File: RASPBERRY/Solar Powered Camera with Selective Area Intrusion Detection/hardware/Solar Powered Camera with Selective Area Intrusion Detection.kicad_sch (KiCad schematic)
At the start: 0 parts

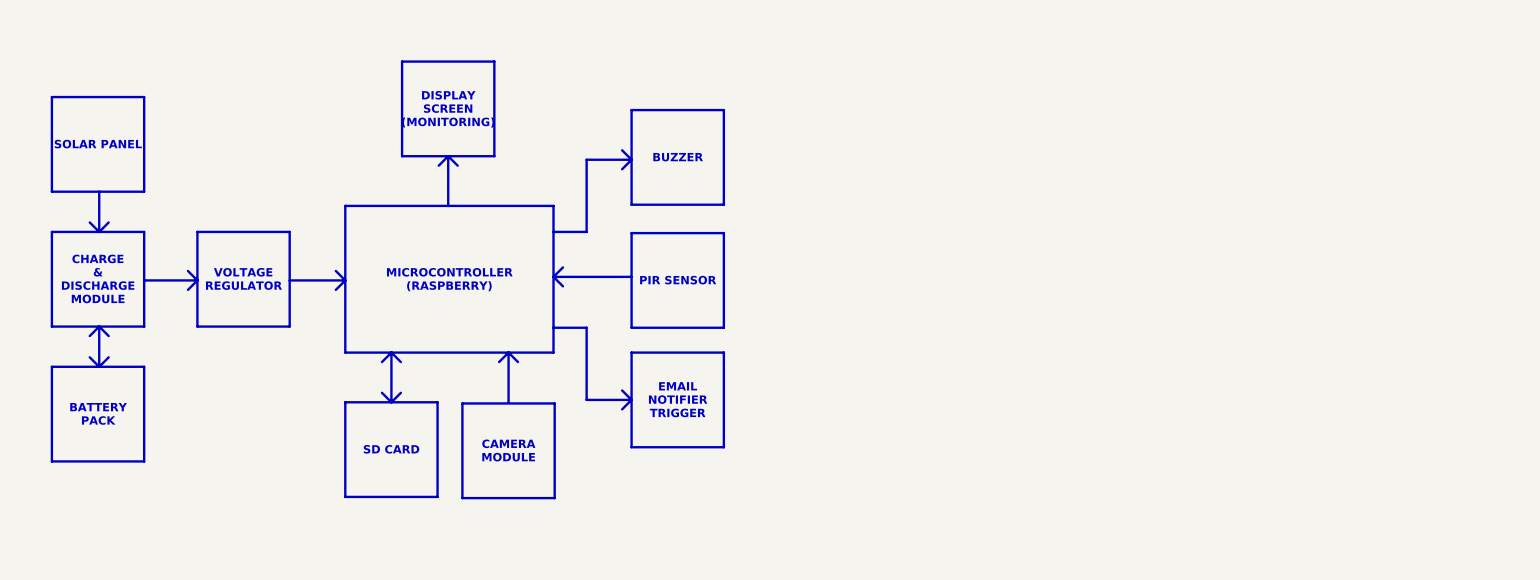
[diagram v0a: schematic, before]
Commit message: update from home
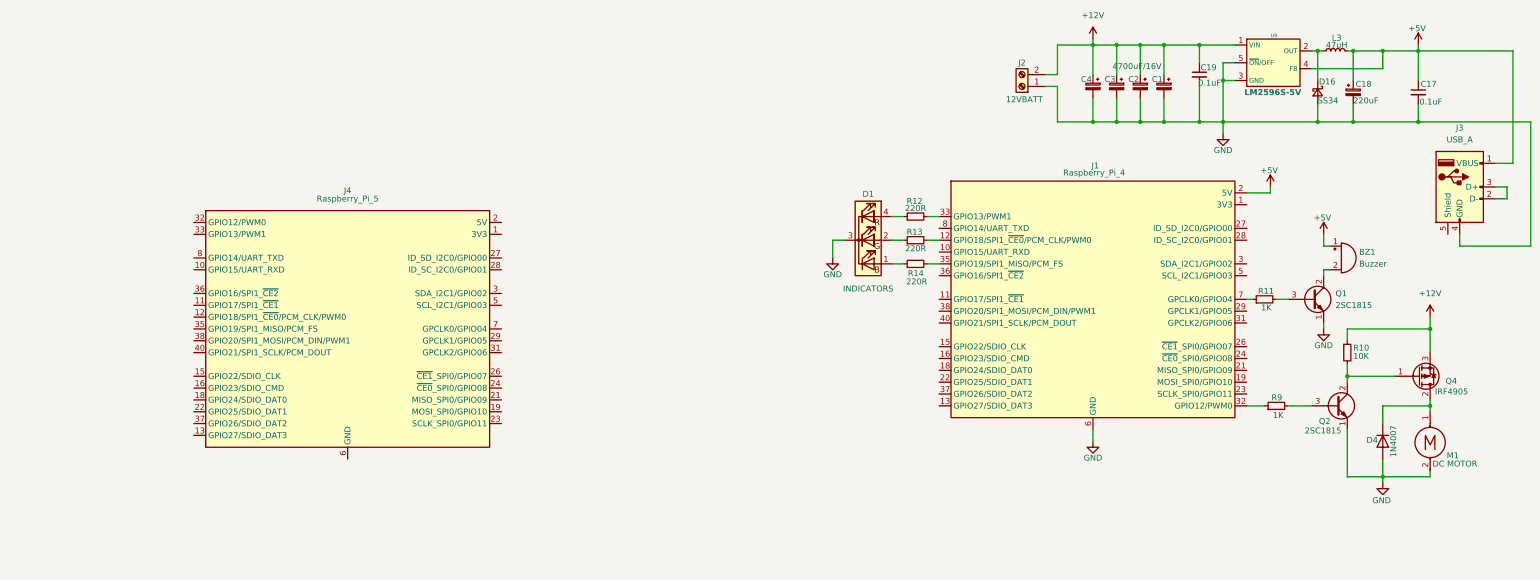
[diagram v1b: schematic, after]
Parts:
- added BZ1: Buzzer, Buzzer_Beeper:Buzzer_12x9.5RM7.6, symbol Device:Buzzer
- added C1: 4700uF/16V, Capacitor_THT:CP_Radial_D13.0mm_P5.00mm, symbol Device:C_Polarized_Small
- added C17, C19: 0.1uF, Capacitor_THT:C_Disc_D7.5mm_W5.0mm_P7.50mm, symbol Device:C_Small
- added C18: 220uF, Capacitor_THT:CP_Radial_D8.0mm_P3.50mm, symbol Device:C_Polarized_Small
- added C2, C3, C4: ~, Capacitor_THT:CP_Radial_D13.0mm_P5.00mm, symbol Device:C_Polarized_Small
- added D1: INDICATORS, LED_THT:LED_D5.0mm-4_RGB, symbol Device:LED_BGKR
- added D16: SS34, Diode_SMD:D_3220_8050Metric, symbol Device:D_Schottky_Small
- added D4: 1N4007, Diode_THT:D_DO-41_SOD81_P10.16mm_Horizontal, symbol Diode:1N4007
- added J1: Raspberry_Pi_4, Connector_PinHeader_2.54mm:PinHeader_2x20_P2.54mm_Vertical, symbol Connector:Raspberry_Pi_4
- added J2: 12VBATT, TerminalBlock_4Ucon:TerminalBlock_4Ucon_1x02_P3.50mm_Vertical, symbol Connector:Screw_Terminal_01x02
- added J3: USB_A, Connector_USB:USB_A_Molex_67643_Horizontal, symbol Connector:USB_A
- added J4: Raspberry_Pi_5, symbol Connector:Raspberry_Pi_4
- added L3: 47uH, Inductor_THT:L_Axial_L14.0mm_D4.5mm_P15.24mm_Horizontal_Fastron_LACC, symbol Device:L_Small
- added M1: DC MOTOR, TerminalBlock_4Ucon:TerminalBlock_4Ucon_1x02_P3.50mm_Vertical, symbol Motor:Motor_AC
- added Q1, Q2: 2SC1815, Package_TO_SOT_THT:TO-92S_Wide, symbol Transistor_BJT:2SC1815
- added Q4: IRF4905, Package_TO_SOT_THT:TO-220-3_Horizontal_TabDown, symbol Transistor_FET:IRF4905
- added R10: 10K, Resistor_THT:R_Axial_DIN0207_L6.3mm_D2.5mm_P10.16mm_Horizontal, symbol Device:R_Small
- added R11, R9: 1K, Resistor_THT:R_Axial_DIN0207_L6.3mm_D2.5mm_P10.16mm_Horizontal, symbol Device:R_Small
- added R12, R13, R14: 220R, Resistor_THT:R_Axial_DIN0207_L6.3mm_D2.5mm_P10.16mm_Horizontal, symbol Device:R_Small
- added U9: LM2596S-5V, Package_TO_SOT_SMD:TO-263-5_TabPin3, symbol Regulator_Switching:LM2596S-ADJ
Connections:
- new net: D16.1 (K), L3.1, U9.2 (OUT)
- new net: Q2.2 (C), Q4.1 (G), R10.2
- new net: J1.7 (GPCLK0/GPIO04), R11.1
- new net: Q1.3 (B), R11.2
- new net: D1.2 (GA), R13.1
- new net: J1.12 (GPIO18/SPI1_~{CE0}/PCM_CLK/PWM0), R13.2
- new net: J1.32 (GPIO12/PWM0), R9.1
- new net: Q2.3 (B), R9.2
- new net: D4.1 (K), M1.1, Q4.2 (D)
- new net: J3.2 (D-), J3.3 (D+)
- new net: BZ1.2 (-), Q1.2 (C)
- new net: D1.4 (RA), R12.1
- new net: J1.33 (GPIO13/PWM1), R12.2
- new net: J1.1 (3V3), J1.17 (3V3)
- new net: J1.35 (GPIO19/SPI1_MISO/PCM_FS), R14.2
- new net: J4.1 (3V3), J4.17 (3V3)
- new net: J4.14 (GND), J4.20 (GND), J4.25 (GND), J4.30 (GND), J4.34 (GND), J4.39 (GND), J4.6 (GND), J4.9 (GND)
- new net: J4.2 (5V), J4.4 (5V)
- new net: D1.1 (BA), R14.1
- new net +12V: C1.1, C19.1, C2.1, C3.1, C4.1, J2.2 (Pin_2), Q4.3 (S), R10.1, U9.1 (VIN)
- new net +5V: BZ1.1 (+), C17.1, C18.1, J1.2 (5V), J1.4 (5V), J3.1 (VBUS), L3.2, U9.4 (FB)
- new net GND: C1.2, C17.2, C18.2, C19.2, C2.2, C3.2, C4.2, D1.3 (K), D16.2 (A), D4.2 (A), J1.14 (GND), J1.20 (GND), J1.25 (GND), J1.30 (GND), J1.34 (GND), J1.39 (GND), J1.6 (GND), J1.9 (GND), J2.1 (Pin_1), J3.4 (GND), M1.2, Q1.1 (E), Q2.1 (E), U9.3 (GND), U9.5 (~{ON}/OFF)

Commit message: UPDATED
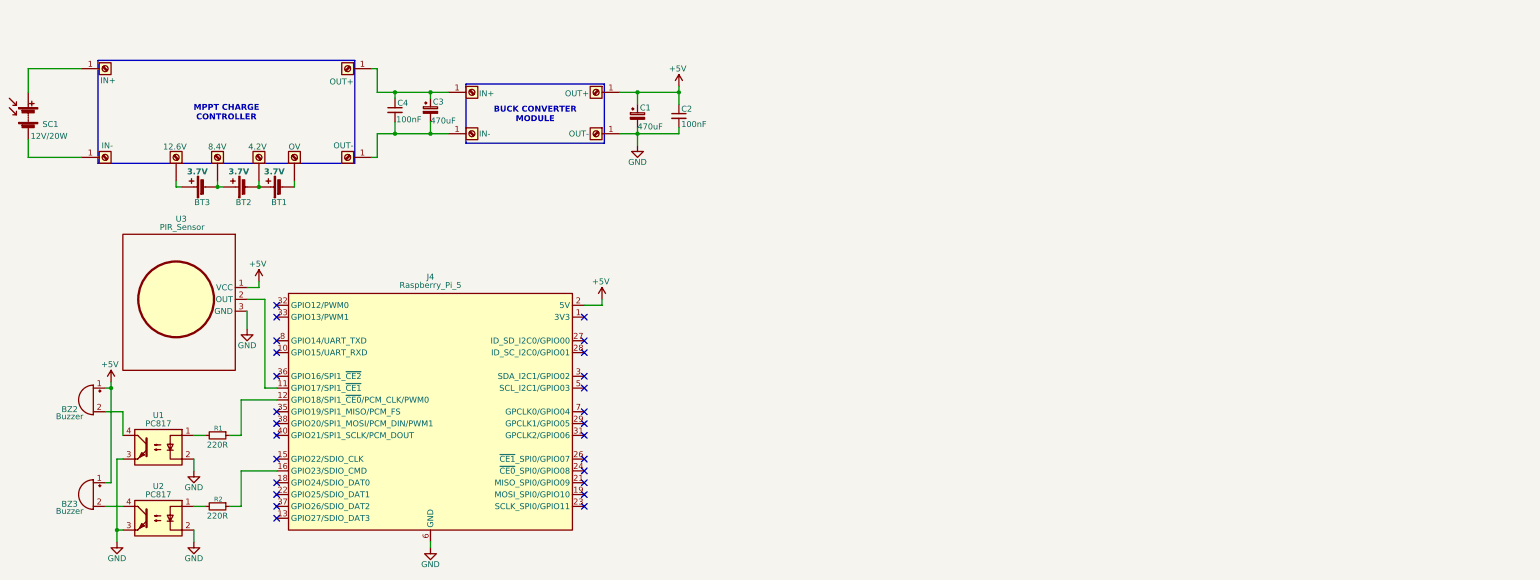
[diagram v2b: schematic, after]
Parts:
- removed BZ1: Buzzer, Buzzer_Beeper:Buzzer_12x9.5RM7.6, symbol Device:Buzzer
- removed C17, C19: 0.1uF, Capacitor_THT:C_Disc_D7.5mm_W5.0mm_P7.50mm, symbol Device:C_Small
- removed C18: 220uF, Capacitor_THT:CP_Radial_D8.0mm_P3.50mm, symbol Device:C_Polarized_Small
- removed C2, C4: ~, Capacitor_THT:CP_Radial_D13.0mm_P5.00mm, symbol Device:C_Polarized_Small
- removed D1: INDICATORS, LED_THT:LED_D5.0mm-4_RGB, symbol Device:LED_BGKR
- removed D16: SS34, Diode_SMD:D_3220_8050Metric, symbol Device:D_Schottky_Small
- removed D4: 1N4007, Diode_THT:D_DO-41_SOD81_P10.16mm_Horizontal, symbol Diode:1N4007
- removed J1: Raspberry_Pi_4, Connector_PinHeader_2.54mm:PinHeader_2x20_P2.54mm_Vertical, symbol Connector:Raspberry_Pi_4
- removed J2: 12VBATT, TerminalBlock_4Ucon:TerminalBlock_4Ucon_1x02_P3.50mm_Vertical, symbol Connector:Screw_Terminal_01x02
- removed J3: USB_A, Connector_USB:USB_A_Molex_67643_Horizontal, symbol Connector:USB_A
- removed L3: 47uH, Inductor_THT:L_Axial_L14.0mm_D4.5mm_P15.24mm_Horizontal_Fastron_LACC, symbol Device:L_Small
- removed M1: DC MOTOR, TerminalBlock_4Ucon:TerminalBlock_4Ucon_1x02_P3.50mm_Vertical, symbol Motor:Motor_AC
- removed Q1, Q2: 2SC1815, Package_TO_SOT_THT:TO-92S_Wide, symbol Transistor_BJT:2SC1815
- removed Q4: IRF4905, Package_TO_SOT_THT:TO-220-3_Horizontal_TabDown, symbol Transistor_FET:IRF4905
- removed R10: 10K, Resistor_THT:R_Axial_DIN0207_L6.3mm_D2.5mm_P10.16mm_Horizontal, symbol Device:R_Small
- removed R11, R9: 1K, Resistor_THT:R_Axial_DIN0207_L6.3mm_D2.5mm_P10.16mm_Horizontal, symbol Device:R_Small
- removed R12, R13, R14: 220R, Resistor_THT:R_Axial_DIN0207_L6.3mm_D2.5mm_P10.16mm_Horizontal, symbol Device:R_Small
- removed U9: LM2596S-5V, Package_TO_SOT_SMD:TO-263-5_TabPin3, symbol Regulator_Switching:LM2596S-ADJ
- added BT1, BT2, BT3: 3.7V, symbol Device:Battery_Cell
- added BZ2, BZ3: Buzzer, symbol Device:Buzzer
- added C2, C4: 100nF, symbol Device:C_Small
- added J1, J6: IN+, symbol Connector:Screw_Terminal_01x01
- added J10: 12.6V, symbol Connector:Screw_Terminal_01x01
- added J11: OV, symbol Connector:Screw_Terminal_01x01
- added J13: 8.4V, symbol Connector:Screw_Terminal_01x01
- added J15: 4.2V, symbol Connector:Screw_Terminal_01x01
- added J2, J7: IN-, symbol Connector:Screw_Terminal_01x01
- added J3, J8: OUT+, symbol Connector:Screw_Terminal_01x01
- added J5, J9: OUT-, symbol Connector:Screw_Terminal_01x01
- added R1, R2: 220R, symbol Device:R_Small
- added SC1: 12V/20W, symbol Device:Solar_Cells
- added U1, U2: PC817, Package_DIP:DIP-4_W7.62mm, symbol Isolator:PC817
- added U3: PIR_Sensor, PCM_SL_Breakout_Boards:PIR-Sensor, symbol PCM_SL_Breakout_Boards:PIR_Sensor
- C1: value 4700uF/16V -> 470uF; footprint Capacitor_THT:CP_Radial_D13.0mm_P5.00mm -> (none)
- C3: value ~ -> 470uF; footprint Capacitor_THT:CP_Radial_D13.0mm_P5.00mm -> (none)
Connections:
- net +5V: now also C1.1, J4.2 (5V), J4.4 (5V), BZ2.1 (+), BZ3.1 (+), C2.1, J8.1 (Pin_1), U3.1 (VCC)
- net GND: now also J4.14 (GND), J4.20 (GND), J4.25 (GND), J4.30 (GND), J4.34 (GND), J4.39 (GND), J4.6 (GND), J4.9 (GND), C2.2, J9.1 (Pin_1), U1.2, U1.3, U2.2, U2.3, U3.3 (GND); no longer C3.2
- net at J4.11 (GPIO17/SPI1_~{CE1}): now also U3.2 (OUT)
- net at J4.12 (GPIO18/SPI1_~{CE0}/PCM_CLK/PWM0): now also R1.1
- net at J4.16 (GPIO23/SDIO_CMD): now also R2.1
- net +12V: no longer names the net of C3.1
- net +12V: now also C4.1, J3.1 (Pin_1), J6.1 (Pin_1); no longer C1.1
- new net: R2.2, U2.1
- new net: BZ3.2 (-), U2.4
- new net: J1.1 (Pin_1), SC1.1 (+)
- new net: J2.1 (Pin_1), SC1.2 (-)
- new net: C3.2, C4.2, J5.1 (Pin_1), J7.1 (Pin_1)
- new net: BT3.1 (+), J10. (Pin_1)
- new net: BT1.2 (-), J11. (Pin_1)
- new net: BT1.1 (+), BT2.2 (-), J15. (Pin_1)
- new net: R1.2, U1.1
- new net: BZ2.2 (-), U1.4
- new net: BT2.1 (+), BT3.2 (-), J13. (Pin_1)
- no-connect marks 0 -> 26
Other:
- moved on the sheet: J4
